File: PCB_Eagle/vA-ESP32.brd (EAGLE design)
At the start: 15 x 35 mm, 65 parts, among them Q4 IRLML6401TR, U1 25Q32, U14 ESP32, U2 LTC4054, U8 LIS3DH, U9 MCP170x-3.0, X3 I2C-SMD-SWATCH-I2C-5, Y1 32.768, Y2 26MHz

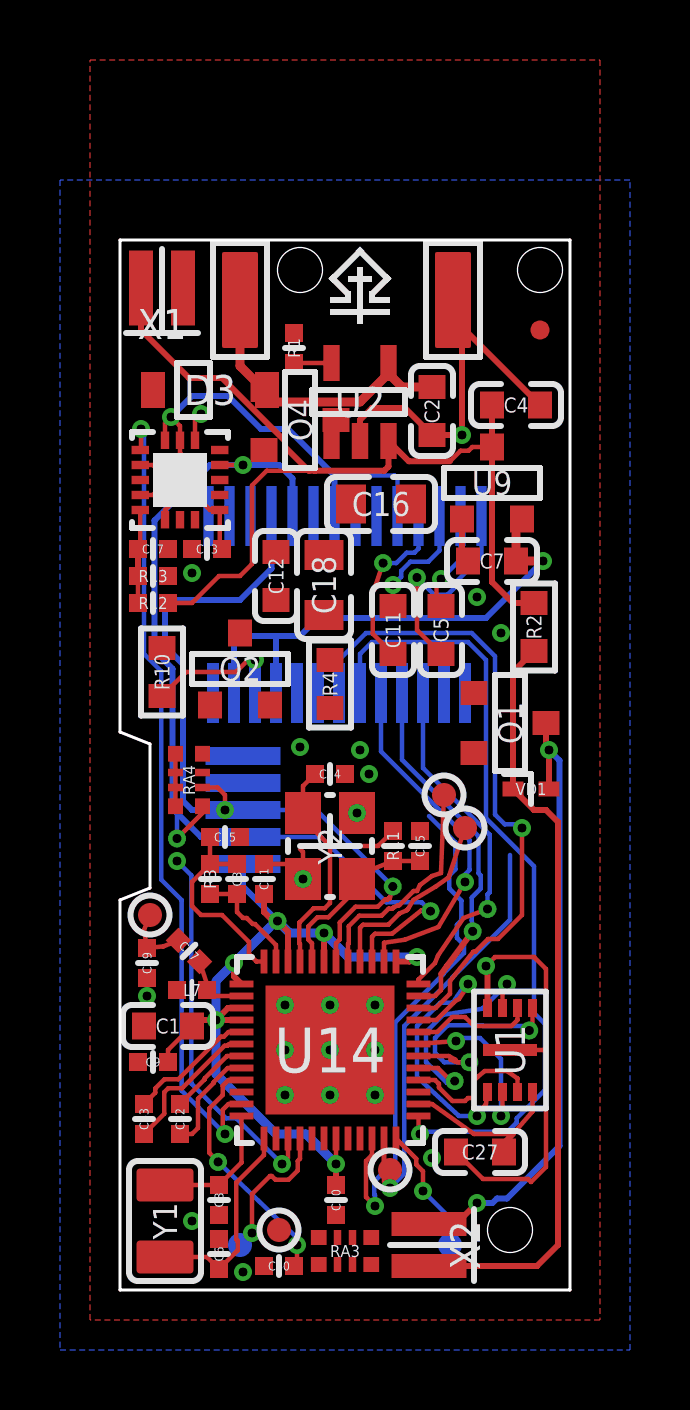
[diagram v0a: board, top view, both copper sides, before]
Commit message: v
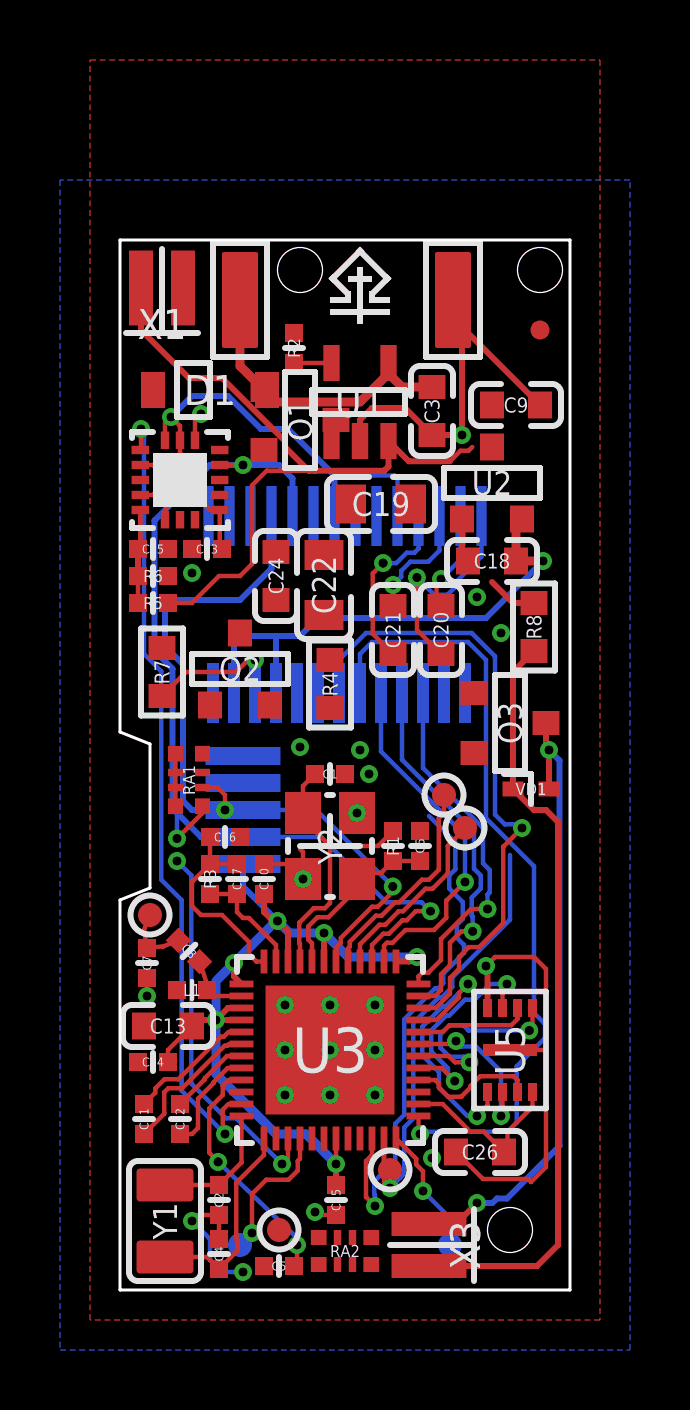
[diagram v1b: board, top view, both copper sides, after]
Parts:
- removed C40, C51: 100nF, !ht3_passive:C0402
- removed C42, C43: 270pF, !ht3_passive:C0402
- removed C47: 3.9pF, !ht3_passive:C0402
- removed C49: 2.4pF, !ht3_passive:C0402
- removed CP10, CP11: (no value), !ht3_connectors:CP-1-C08MM
- removed Q4: IRLML6401TR, !ht3_transistor:SOT23-3-1
- removed R11: 1M/10%, !ht3_passive:R0402
- removed U9: MCP170x-3.0, !ht3_ic:SOT23-3
- added C19: 2.2uFx16V, !ht3_passive:C0805
- added C20, C21: 1uFx16V, !ht3_passive:C0603
- added C22: 4.7uFx16V, !ht3_passive:C0805
- added C23: 1uF, !ht3_passive:C0402
- added C24: 100nF, !ht3_passive:C0603
- added CP5, CP6: (no value), !ht3_connectors:CP-1-C08MM
- added Q3: (no value), !ht3_transistor:SOT23-3-1
- added R8: 100, !ht3_passive:R0603
- added U5: 25Q32, !ht3_ic:USON-8-2X3
- C1: value 100nF -> 10pF; device !ht3_passive:C0603 -> !ht3_passive:C0402
- C11: device !ht3_passive:C0603 -> !ht3_passive:C0402
- C12: value 100nF -> 270pF; device !ht3_passive:C0603 -> !ht3_passive:C0402
- C13: value 1uF -> 100nF; device !ht3_passive:C0402 -> !ht3_passive:C0603
- C14, C15: value 10pF -> 100nF
- C16: value 270pF -> 10nF; device !ht3_passive:C0805 -> !ht3_passive:C0402
- C17: value 100nF -> 3nF
- C18: value 270pF -> 4.7uF; device !ht3_passive:C0805 -> !ht3_passive:C0603
- C2, C4: value 4.7uF -> 10pF; device !ht3_passive:C0603 -> !ht3_passive:C0402
- C25: value 10nF -> 100nF
- C3: value 3nF -> 4.7uF; device !ht3_passive:C0402 -> !ht3_passive:C0603
- C5: value 270pF -> 100nF; device !ht3_passive:C0603 -> !ht3_passive:C0402
- C7: value 4.7uF -> 2.4pF; device !ht3_passive:C0603 -> !ht3_passive:C0402
- C8: value 10pF -> 3.9pF
- C9: value 100nF -> 4.7uF; device !ht3_passive:C0402 -> !ht3_passive:C0603
- CP1: device !ht3_connectors:CP-1-C08MM -> !ht3_connectors:CP-1-R08MM
- CP3: device !ht3_connectors:CP-1-R08MM -> !ht3_connectors:CP-1-C08MM
- Q1: value (none) -> IRLML6401TR
- R1: value 10K -> 1M/10%
- R2: value 100 -> 10K; device !ht3_passive:R0603 -> !ht3_passive:R0402
- R4: value 560K -> 390-560K
- R6: value 100K -> 1M
- U1: value 25Q32 -> LTC4054; device !ht3_ic:USON-8-2X3 -> !ht3_ic:SOT23-5L
- U2: value LTC4054 -> MCP170x-3.0; device !ht3_ic:SOT23-5L -> !ht3_ic:SOT23-3
- X2: value (none) -> I2C-SMD-SWATCH-I2C-5; device !ht3_connectors:2C_SMD-SWATCH -> !ht3_connectors:SMD-SWATCH-I2C-5
- X3: value I2C-SMD-SWATCH-I2C-5 -> (none); device !ht3_connectors:SMD-SWATCH-I2C-5 -> !ht3_connectors:2C_SMD-SWATCH
- moved CP1 32.3 mm to (11.1, 33.0), flipped to the top
- moved C4 30.0 mm to (3.30, 1.20), turned to 90 degrees
- moved C2 27.2 mm to (3.30, 3.00)
- moved C9 25.0 mm to (13.2, 29.5), turned to 0 degrees
- moved U1 22.2 mm to (8.00, 29.6), turned to 0 degrees
- moved C5 21.9 mm to (5.30, 0.80), turned to 180 degrees
- moved CP3 20.7 mm to (1.00, 12.5), turned to 180 degrees
- moved C12 18.4 mm to (2.00, 5.70)
- moved C11 18.3 mm to (0.80, 5.70), turned to 270 degrees
- moved C7 17.7 mm to (0.90, 10.9), turned to 270 degrees
- moved R1 16.9 mm to (9.10, 14.8), turned to 270 degrees
- moved C3 16.9 mm to (10.4, 29.3), turned to 270 degrees
- moved CP7 16.5 mm to (4.00, 1.50), flipped to the bottom, turned to 0 degrees
- moved X2 16.3 mm to (4.10, 16.0), flipped to the bottom, turned to 90 degrees
- moved X3 16.3 mm to (11.5, 1.50), flipped to the top, turned to 0 degrees
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- renumbered C27 to C26, D3 to D1, L7 to L1, R10 to R7, R12 to R5, R13 to R6, RA3 to RA2, RA4 to RA1, U14 to U3, U8 to U4
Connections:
- removed net VBAT1: Q4.3
- new net N$13: D1.C, Q1.2, U2.3
- net +5V: now also C3.1, CP2.1, Q1.1, U1.4; no longer C2.1, CP3.1, Q4.1, U2.4
- net ANT: now also C7.1, C8.1, CP3.1; no longer C47.1, C49.1, CP4.1
- net EN: now also C5.1, CP8.1; no longer C40.1, CP10.1
- net GND: now also C19.2, C22.2, C23.2, C24.2, C3.2, C5.2, CP1.1, Q3.2, R2.2, U1.2, U2.1, U5.4, U5.P$1, X2.5; no longer C12.2, C17.2, C40.2, C49.2, C51.2, C8.2, CP2.1, Q1.2, R1.2, U1.4, U1.P$1, U2.2, U9.1, X3.5
- net I2C_SCL: now also X2.2; no longer X3.2
- net I2C_SDA: now also X2.3; no longer X3.3
- net I36: now also C11.1; no longer C43.1
- net I37: now also C11.2; no longer C43.2
- net I38: now also C12.1; no longer C42.1
- net I39: now also C12.2; no longer C42.2
- net IO0: now also CP9.1; no longer CP11.1
- net IO1: now also CP4.1; no longer CP7.1
- net IO10: now also U5.3; no longer U1.3
- net IO11: now also U5.1; no longer U1.1
- net IO27: now also CP7.1; no longer CP1.1
- net IO3: now also CP5.1; no longer CP8.1
- net IO4: now also CP6.1; no longer CP9.1
- net IO6: now also U5.6; no longer U1.6
- net IO7: now also U5.2; no longer U1.2
- net IO8: now also U5.5; no longer U1.5
- net IO9: now also U5.7; no longer U1.7
- net MOTOR: now also Q3.1; no longer Q1.1
- net N$1: now also C21.2; no longer C11.2
- net N$10: now also C20.2; no longer C5.2
- net N$11: now also C22.1, C24.1; no longer C12.1, C18.1
- net N$12: now also C19.1; no longer C16.1
- net N$2: now also C17.1; no longer C3.1
- net N$22: now also Q3.3, X3.2; no longer Q1.3, X2.2
- net N$23: now also R8.2, X3.1; no longer R2.2, X2.1
- net N$3: now also C21.1; no longer C11.1
- net N$4: now also C16.1, C17.2; no longer C25.1, C3.2
- net N$5: now also C20.1; no longer C5.1
- net N$6: now also R2.1, U1.5; no longer R1.1, U2.5
- net N$7: now also C8.2; no longer C47.2
- net OSC26_I: now also C1.1, R1.1; no longer C14.1, R11.1
- net OSC26_O: now also C6.1, R1.2; no longer C15.1, R11.2
- net OSC32_I: now also C2.1; no longer C8.1
- net OSC32_O: now also C4.1; no longer C6.1
- net VBAT: now also C9.1, Q1.3, R8.1, U1.3; no longer C4.1, D1.C, Q4.2, R2.1, U2.3, U9.3
- net VBAT_ADC: now also C25.1; no longer C17.1
- net VDD: now also C14.1, C15.1, C18.1, C23.1, U2.2, X2.1; no longer C1.1, C51.1, C7.1, C9.1, U9.2, X3.1
- net VDD_SDIO: now also U5.8; no longer U1.8
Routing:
- net VBAT: track 32.4 -> 25.8 mm
- net GND: track 34.7 -> 40.0 mm, vias 24 -> 25
- net IO11: track 8.11 -> 7.36 mm
- net IO9: track 4.94 -> 4.37 mm

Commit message: v
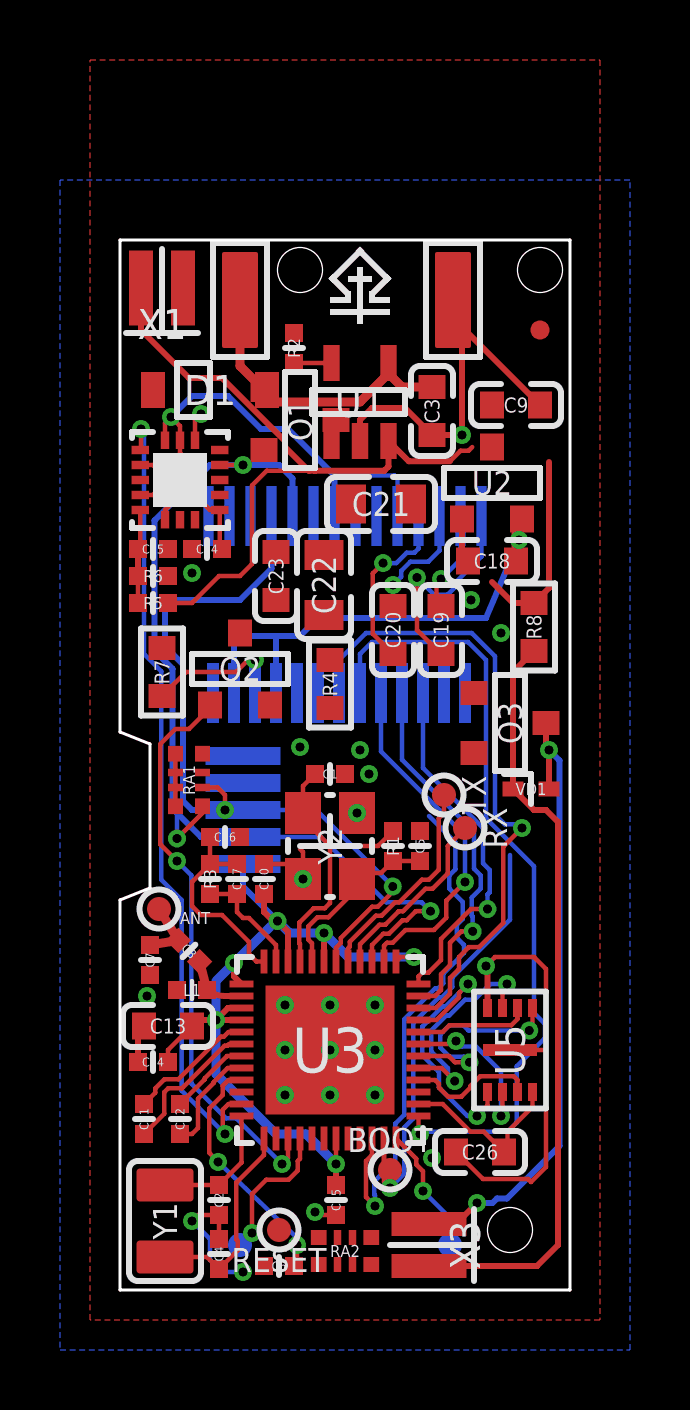
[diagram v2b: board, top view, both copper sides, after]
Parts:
- C19: value 2.2uFx16V -> 1uFx16V; device !ht3_passive:C0805 -> !ht3_passive:C0603
- C2, C4: value 10pF -> 12pF
- C21: value 1uFx16V -> 2.2uFx16V; device !ht3_passive:C0603 -> !ht3_passive:C0805
- C23: value 1uF -> 100nF; device !ht3_passive:C0402 -> !ht3_passive:C0603
- C24: value 100nF -> 1uF; device !ht3_passive:C0603 -> !ht3_passive:C0402
- C5: value 100nF -> 10pF
- C6: value 10pF -> 100nF
- CP1: value (none) -> GND
- CP2: value (none) -> +5V
- CP3: value (none) -> ANT
- CP4: value (none) -> TX
- CP5: value (none) -> RX
- CP6: value (none) -> TL
- CP7: value (none) -> TR
- CP8: value (none) -> RESET
- CP9: value (none) -> BOOT
- D1: value SS34 -> NF
- Q2, Q3: value (none) -> IRLML0030
- R7, R8: value 100 -> 10
- U2: value MCP170x-3.0 -> MCP170x-3.3
- VD1: value (none) -> 4148
- X1, X3: value (none) -> PCB
- moved C5 14.8 mm to (10.0, 14.8), turned to 90 degrees
- moved C6 14.8 mm to (5.30, 0.80), turned to 180 degrees
- moved C19 4.65 mm to (10.7, 22.0), turned to 270 degrees
- moved C21 4.22 mm to (8.70, 26.2), turned to 0 degrees
- moved C23 2.47 mm to (5.20, 23.8), turned to 270 degrees
- moved C24 2.47 mm to (2.90, 24.7), turned to 180 degrees
- moved C20 1.60 mm to (9.10, 22.0), turned to 90 degrees
- moved CP3 0.36 mm to (1.30, 12.7)
- moved C7 0.14 mm to (1.00, 11.0)
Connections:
- removed net /INT: RA1.3
- removed net IO17: U3.27
- removed net IO25: U3.14
- removed net JTAG_TCK: U3.20
- removed net JTAG_TDI: U3.18
- removed net JTAG_TDO: U3.21
- removed net JTAG_TMS: U3.17
- removed net MOTOR: Q3.1, U3.15
- new net IO26: Q2.1, RA2.3, U3.15
- net /IRQ: now also RA1.3
- net EN: now also C6.1, RA2.4; no longer C5.1, RA2.1
- net GND: now also C21.2, RA2.8; no longer C19.2
- net IO2: now also Q3.1, RA2.1; no longer Q2.1, RA2.3
- net N$1: now also C20.2; no longer C21.2
- net N$10: now also C19.2; no longer C20.2
- net N$11: now also C23.1; no longer C24.1
- net N$12: now also C21.1; no longer C19.1
- net N$13: now also C9.1
- net N$3: now also C20.1; no longer C21.1
- net N$5: now also C19.1; no longer C20.1
- net OSC26_O: now also C5.1; no longer C6.1
- net VBAT: no longer C9.1
- net VDD: now also C24.1, RA2.5; no longer C23.1, RA2.7, RA2.8
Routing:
- net IO26: track 0.00 -> 19.1 mm, vias 0 -> 2
- net MOTOR: track 12.7 -> 0.00 mm, vias 2 -> 0
- net VBAT: track 25.8 -> 30.7 mm
- net GND: track 40.0 -> 41.3 mm

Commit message: v
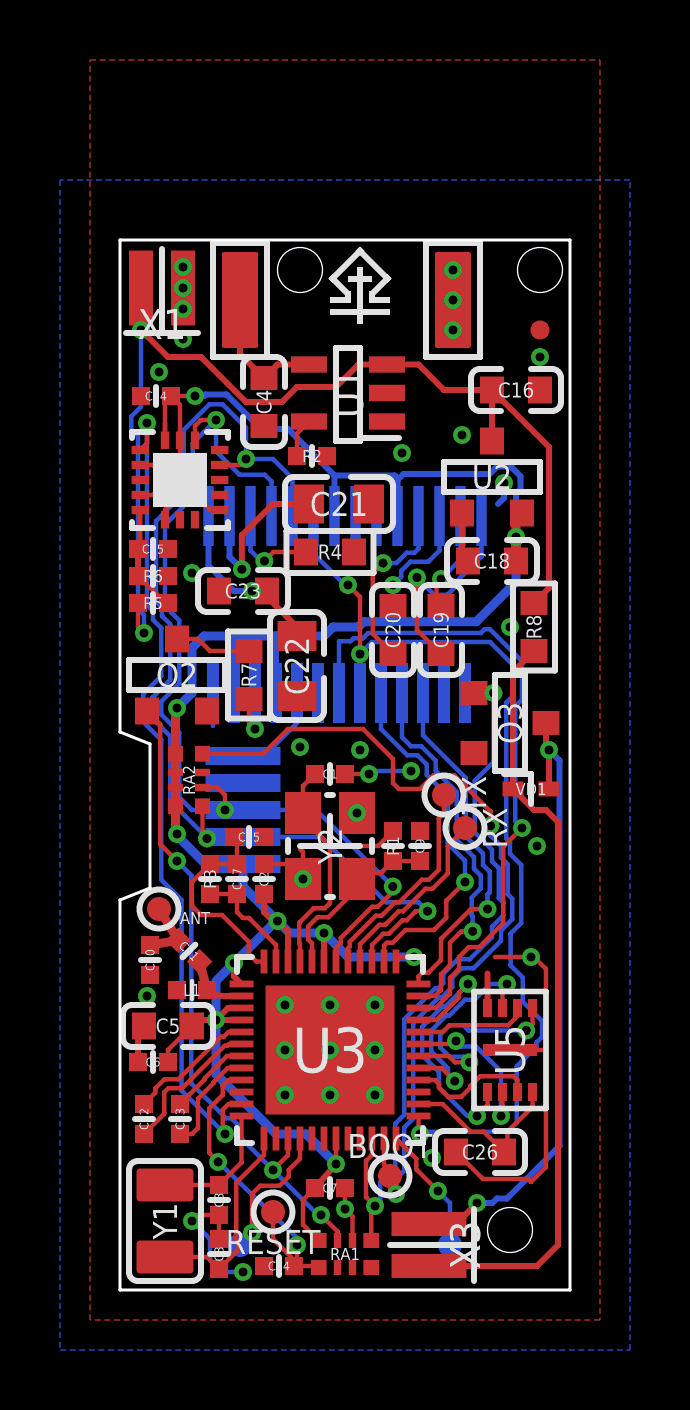
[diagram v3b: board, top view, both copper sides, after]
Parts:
- removed D1: NF, !ht3_diode:SOD123
- removed Q1: IRLML6401TR, !ht3_transistor:SOT23-3-1
- C10: value 100nF -> 2.4pF
- C11: value 270pF -> 3.9pF
- C13: value 100nF -> 270pF; device !ht3_passive:C0603 -> !ht3_passive:C0402
- C15: value 100nF -> 10nF
- C16: value 10nF -> 4.7uF; device !ht3_passive:C0402 -> !ht3_passive:C0603
- C2: value 12pF -> 100nF
- C3: value 4.7uF -> 12pF; device !ht3_passive:C0603 -> !ht3_passive:C0402
- C4: value 12pF -> 4.7uF; device !ht3_passive:C0402 -> !ht3_passive:C0603
- C5: value 10pF -> 100nF; device !ht3_passive:C0402 -> !ht3_passive:C0603
- C7: value 2.4pF -> 100nF
- C8: value 3.9pF -> 12pF
- C9: value 4.7uF -> 10pF; device !ht3_passive:C0603 -> !ht3_passive:C0402
- moved C4 28.4 mm to (4.80, 29.6), turned to 270 degrees
- moved C3 27.2 mm to (3.30, 3.00)
- moved C16 17.8 mm to (13.2, 30.0)
- moved RA1 16.6 mm to (7.50, 1.20), turned to 180 degrees
- moved RA2 16.5 mm to (2.30, 17.0), turned to 90 degrees
- moved C9 15.0 mm to (10.0, 14.8), turned to 90 degrees
- moved C15 12.4 mm to (4.30, 15.1), turned to 0 degrees
- moved C2 10.8 mm to (4.80, 13.7), turned to 90 degrees
- moved C5 10.3 mm to (1.60, 8.80), turned to 180 degrees
- moved C8 10.1 mm to (3.30, 1.20), turned to 90 degrees
- moved C7 9.68 mm to (7.00, 3.40), turned to 0 degrees
- moved C14 7.99 mm to (5.30, 0.80)
- moved C6 7.99 mm to (1.10, 7.60)
- moved C11 5.80 mm to (2.30, 11.3), turned to 315 degrees
- moved C24 5.38 mm to (1.20, 29.8)
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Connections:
- removed net N$13: C9.1, D1.C, Q1.2, U2.3
- net +5V: now also C4.1; no longer C3.1, D1.A, Q1.1
- net /IRQ: no longer RA1.3
- net ANT: now also C10.1, C11.1; no longer C7.1, C8.1
- net EN: now also C14.1, RA1.5; no longer C6.1, RA2.4
- net GND: now also C8.2, RA1.2, RA1.6, RA1.7, RA1.8; no longer C13.2, RA2.6, RA2.8
- net I2C_SCL: now also RA2.1; no longer RA1.1
- net I2C_SDA: now also RA2.2; no longer RA1.2
- net I36: now also C12.1; no longer C11.1
- net I37: now also C12.2; no longer C11.2
- net I38: now also C13.1; no longer C12.1
- net I39: now also C13.2; no longer C12.2
- net IO0: now also RA2.4; no longer RA1.4
- net IO2: now also RA1.1; no longer RA2.1
- net IO26: now also RA1.3; no longer RA2.3
- net N$4: now also C15.1; no longer C16.1
- net N$7: now also C11.2; no longer C8.2
- net OSC26_O: now also C9.1; no longer C5.1
- net OSC32_I: now also C3.1; no longer C2.1
- net OSC32_O: now also C8.1; no longer C4.1
- net VBAT: now also C16.1, U2.3; no longer Q1.3
- net VDD: now also C2.1, C5.1, C6.1, C7.1, RA1.4, RA2.6, RA2.7, RA2.8; no longer C10.1, C13.1, C14.1, C15.1, RA1.5, RA1.6, RA1.7, RA1.8
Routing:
- net VDD: track 70.4 -> 89.3 mm, vias 8 -> 10
- net IO0: track 15.7 -> 28.9 mm, vias 1 -> 2
- net IO2: track 17.7 -> 24.1 mm, vias 1 -> 2
- net I2C_SDA: track 26.6 -> 32.8 mm
- net SCREEN_RES: track 26.5 -> 32.7 mm, vias 1 -> 3
- net N$11: track 0.00 -> 5.87 mm, vias 0 -> 1
- net N$12: track 0.00 -> 5.75 mm, vias 0 -> 1
- net VBAT: track 30.7 -> 36.3 mm, vias 0 -> 2
- net +5V: track 10.0 -> 4.62 mm
- net GND: track 41.3 -> 35.9 mm, vias 25 -> 37
- net N$14: track 0.00 -> 3.27 mm, vias 0 -> 1
- net EN: track 8.28 -> 11.3 mm
- net I2C_SCL: track 32.7 -> 35.4 mm
- net IO26: track 19.1 -> 21.7 mm, vias 2 -> 3
- net N$9: track 0.00 -> 2.57 mm
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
